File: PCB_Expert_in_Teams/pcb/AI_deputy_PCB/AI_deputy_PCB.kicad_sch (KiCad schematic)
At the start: 23 parts, among them J1 Piezo Electric, J3 Haptic Power and GND, J4 UART, J5 JST CONN from MCU, J6 JTAG, Q1 NMOS, SW1 BOOT SWITCH, SW2 RESET SWITCH, U2 ESP32-WROOM-32UE

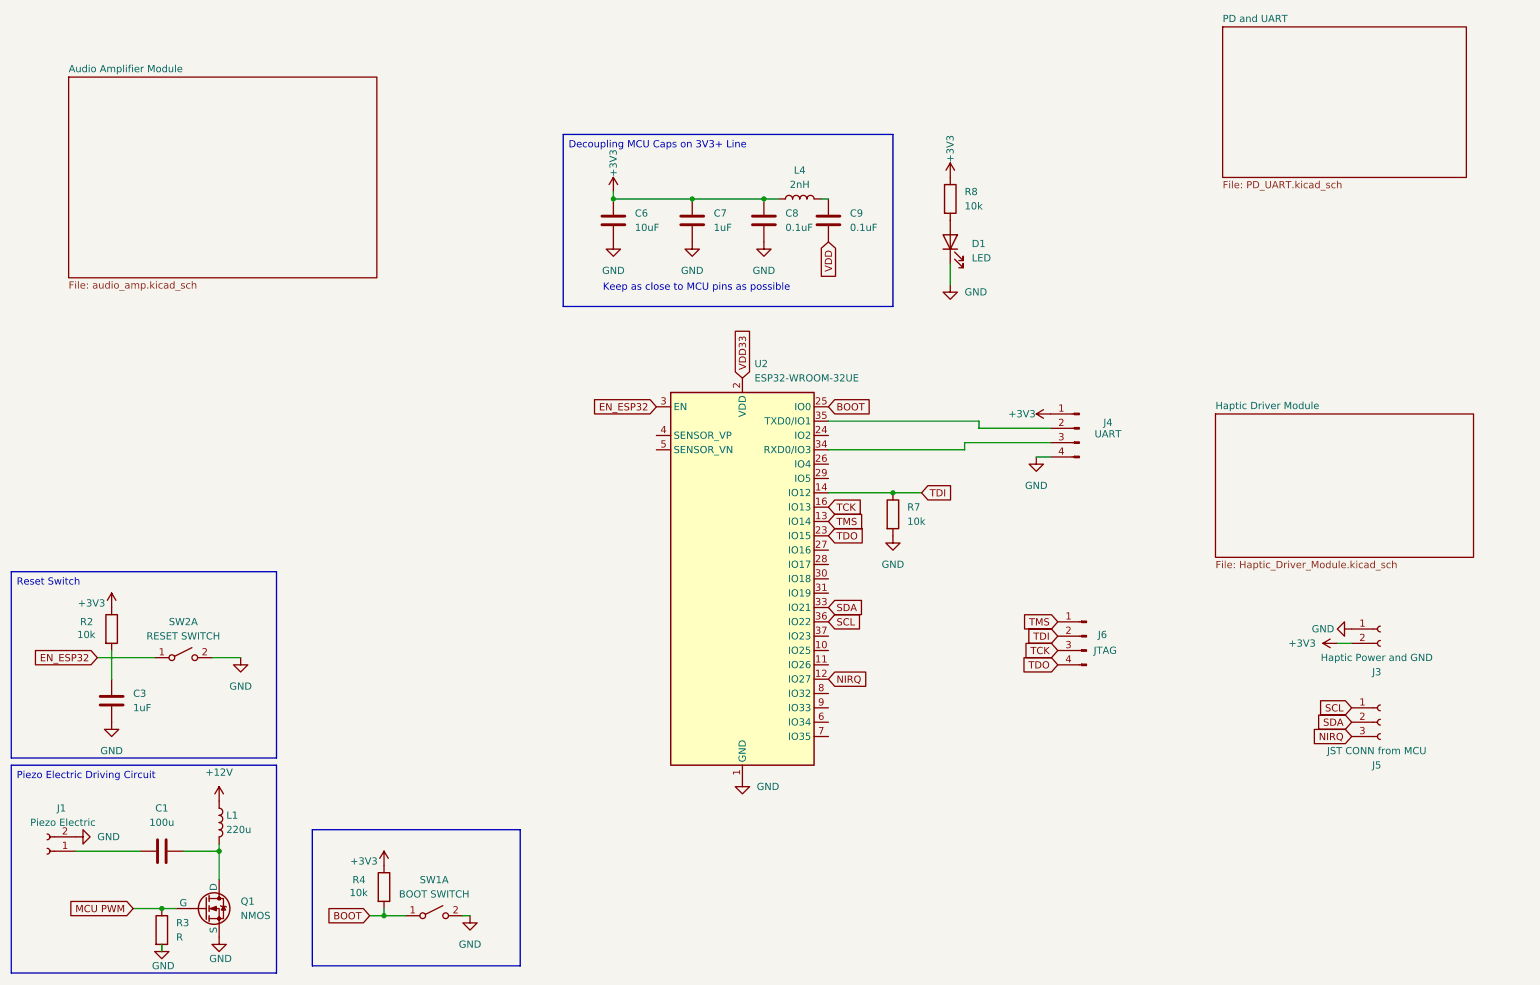
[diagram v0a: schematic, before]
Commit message: progress on PCB + matlab calculations
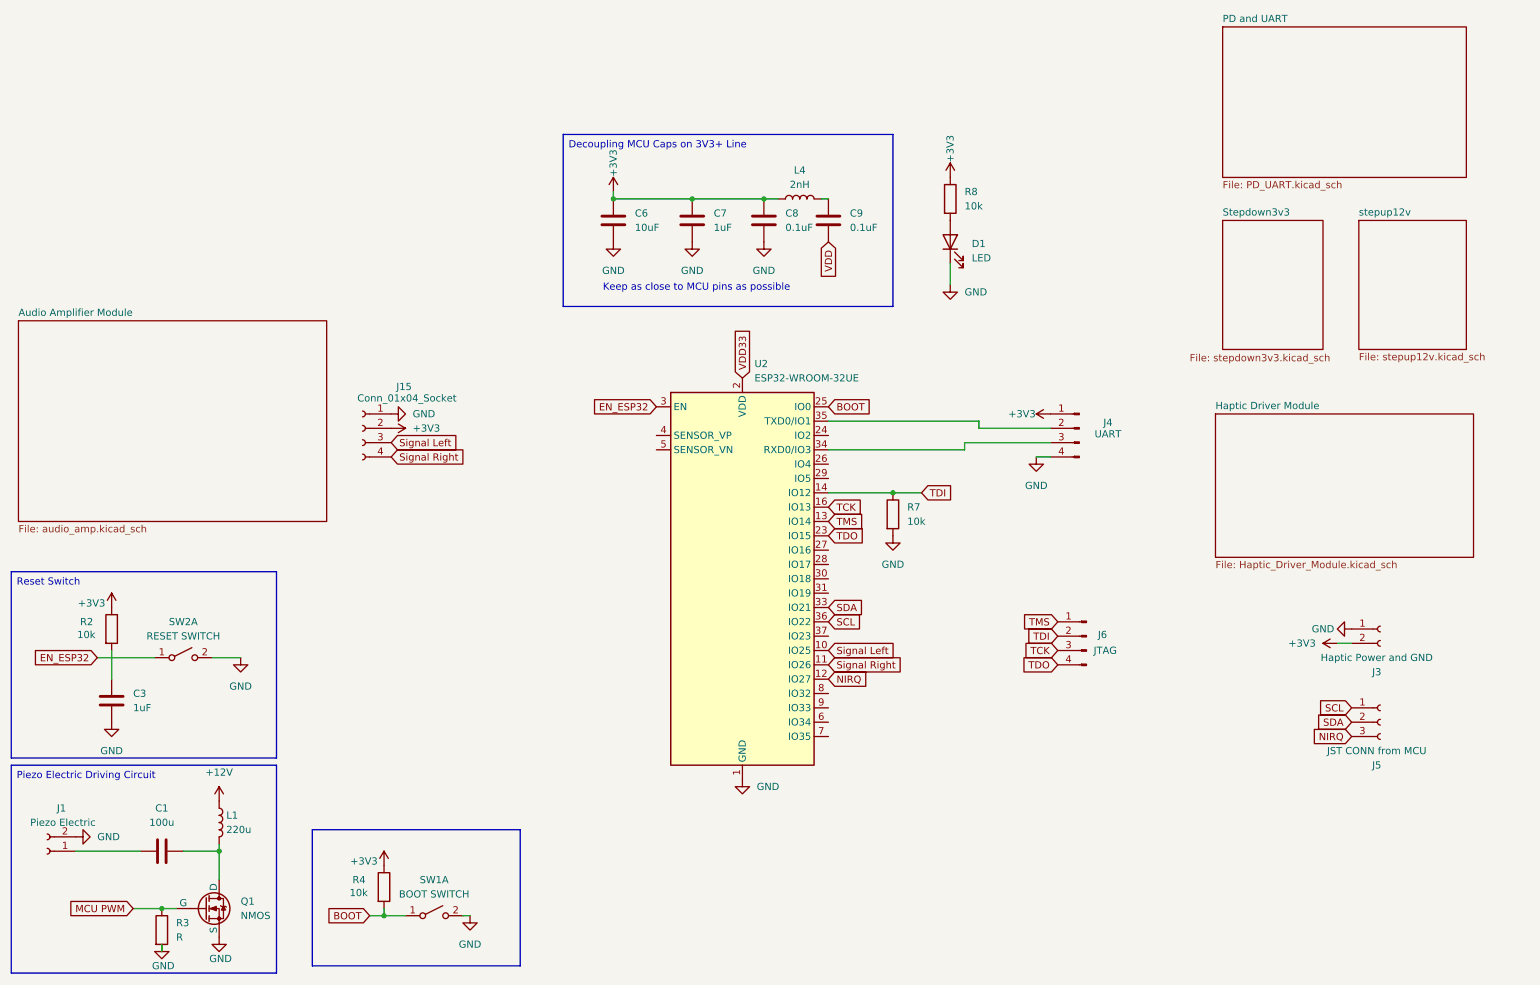
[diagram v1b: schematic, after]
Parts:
- added J15: Conn_01x04_Socket, symbol Connector:Conn_01x04_Socket
- J1: footprint Connector_JST:JST_XH_B1B-XH-AM_1x01_P2.50mm_Vertical -> Connector_JST:JST_XH_S2B-XH-A-1_1x02_P2.50mm_Horizontal
- Q1: footprint (none) -> Package_TO_SOT_SMD:TO-252-3_TabPin2
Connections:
- net +3V3: now also J15.2 (Pin_2)
- net GND: now also J15.1 (Pin_1)
- net Signal Left: now reaches U2.10 (IO25)
- net Signal Left: now also J15.3 (Pin_3)
- net Signal Right: now reaches U2.11 (IO26)
- net Signal Right: now also J15.4 (Pin_4)
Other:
- added sheet Stepdown3v3 (stepdown3v3.kicad_sch)
- added sheet stepup12v (stepup12v.kicad_sch)
